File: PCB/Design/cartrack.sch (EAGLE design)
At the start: 1 part

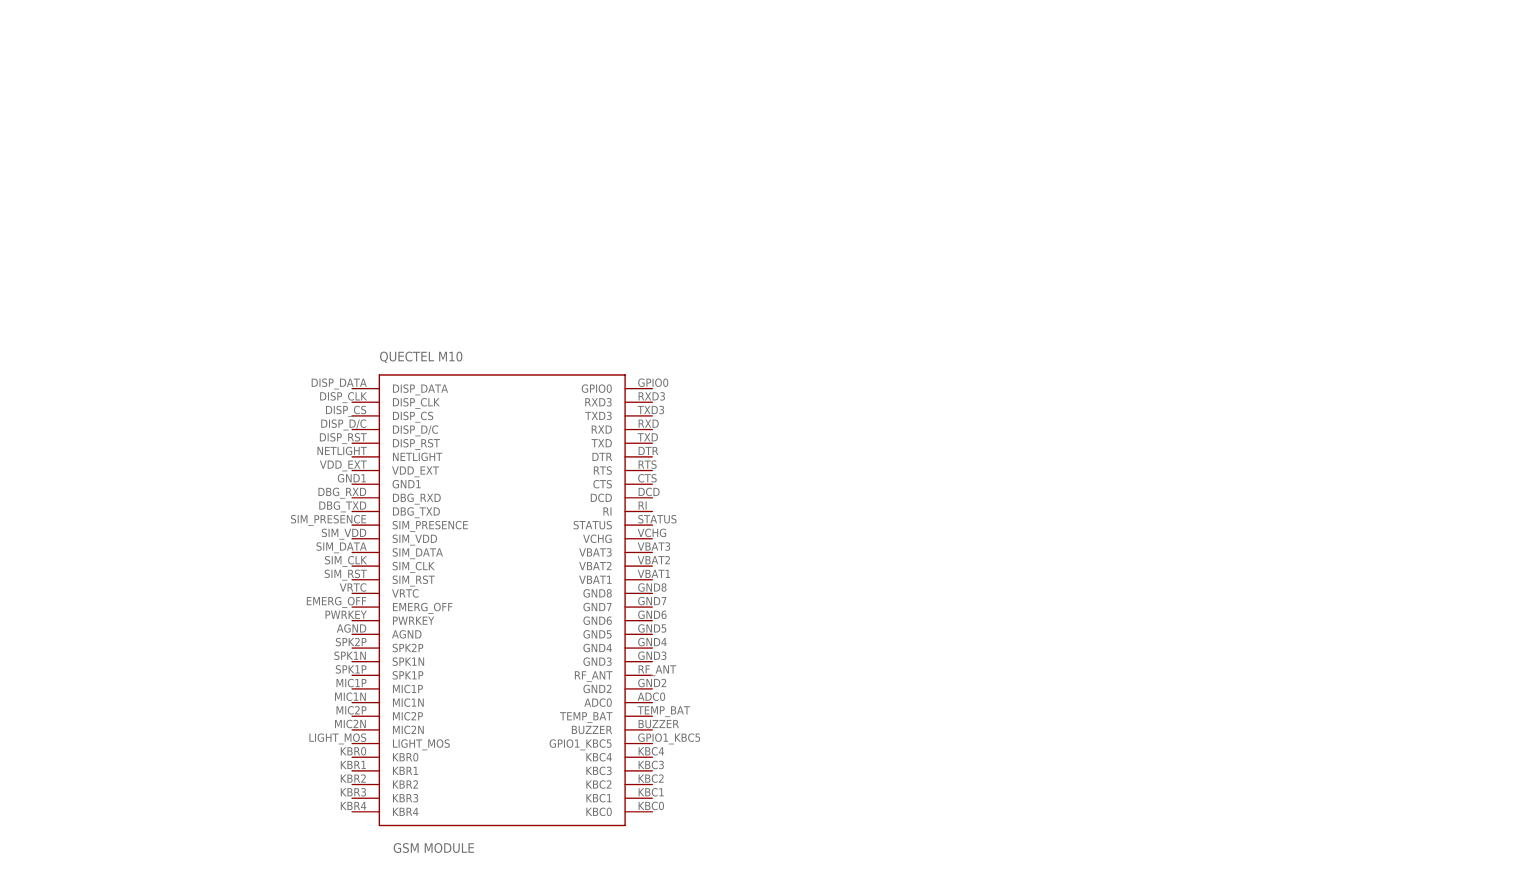
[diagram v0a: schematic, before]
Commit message: Done most of the GSM schematic.
Power and GPS remain
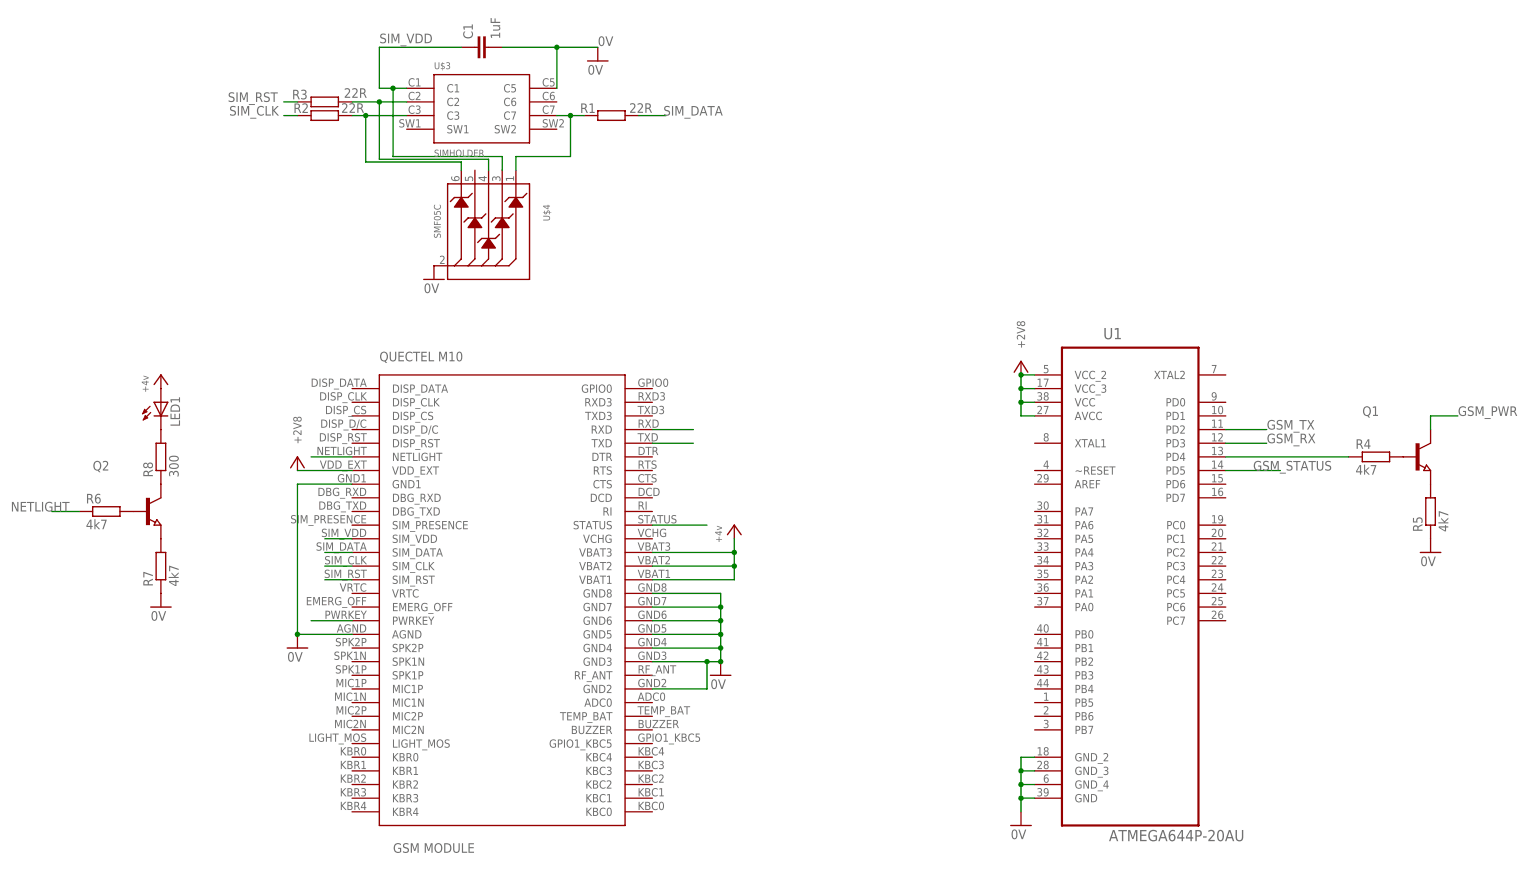
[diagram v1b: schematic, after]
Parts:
- added C1: 1uF, resistor:C-EUC0603
- added LED1: (no value), led:LEDSML0603
- added Q1, Q2: (no value), semicon-smd-ipc:NPN-TRANSISTOR_SOT23W
- added R1, R2, R3: 22R, resistor:R-EU_R0603
- added R4, R5, R6, R7: 4k7, resistor:R-EU_R0603
- added R8: 300, resistor:R-EU_R0603
- added U$3: SIMHOLDER, SparkFun-Connectors:SIMHOLDER
- added U$4: SMF05C, Simplex-DiscreteSemi:SMF05C
- added U1: ATMEGA644P-20AU, Atmel_By_element14_Batch_1:ATMEGA644P-20AU
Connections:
- new net +2V8: U$1.VDD_EXT, U1.AVCC, U1.VCC, U1.VCC_2, U1.VCC_3
- new net +4V: LED1.A, U$1.VBAT1, U$1.VBAT2, U$1.VBAT3
- new net 0V: C1.2, R5.1, R7.1, U$1.AGND, U$1.GND1, U$1.GND2, U$1.GND3, U$1.GND4, U$1.GND5, U$1.GND6, U$1.GND7, U$1.GND8, U$3.C5, U$4.ANODE, U1.GND, U1.GND_2, U1.GND_3, U1.GND_4
- new net GSM_PWR: Q1.C, U$1.PWRKEY
- new net GSM_RX: U$1.RXD, U1.PD3
- new net GSM_STATUS: U$1.STATUS, U1.PD5
- new net GSM_TX: U$1.TXD, U1.PD2
- new net N$1: R1.1, U$3.C7, U$4.CATODE1
- new net N$10: LED1.C, R8.2
- new net N$2: R2.2, U$3.C3, U$4.CATODE5
- new net N$3: R3.2, U$3.C2, U$4.CATODE3
- new net N$4: Q1.E, R5.2
- new net N$5: Q1.B, R4.2
- new net N$6: R4.1, U1.PD4
- new net N$7: Q2.E, R7.2
- new net N$8: Q2.B, R6.2
- new net N$9: Q2.C, R8.1
- new net NETLIGHT: R6.1, U$1.NETLIGHT
- new net SIM_CLK: R2.1, U$1.SIM_CLK
- new net SIM_DATA: R1.2, U$1.SIM_DATA
- new net SIM_RST: R3.1, U$1.SIM_RST
- new net SIM_VDD: C1.1, U$1.SIM_VDD, U$3.C1, U$4.CATODE2
